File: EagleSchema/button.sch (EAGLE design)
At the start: 38 parts, among them IC1 TP4056

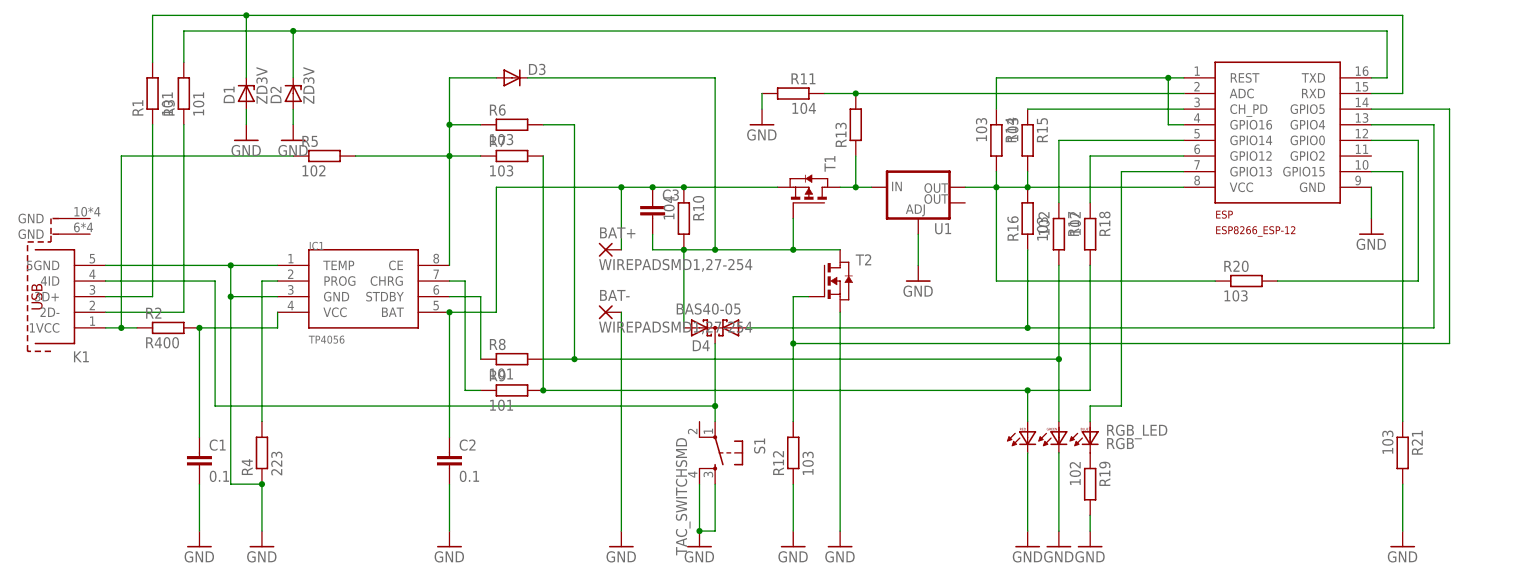
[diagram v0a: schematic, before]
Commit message: new version
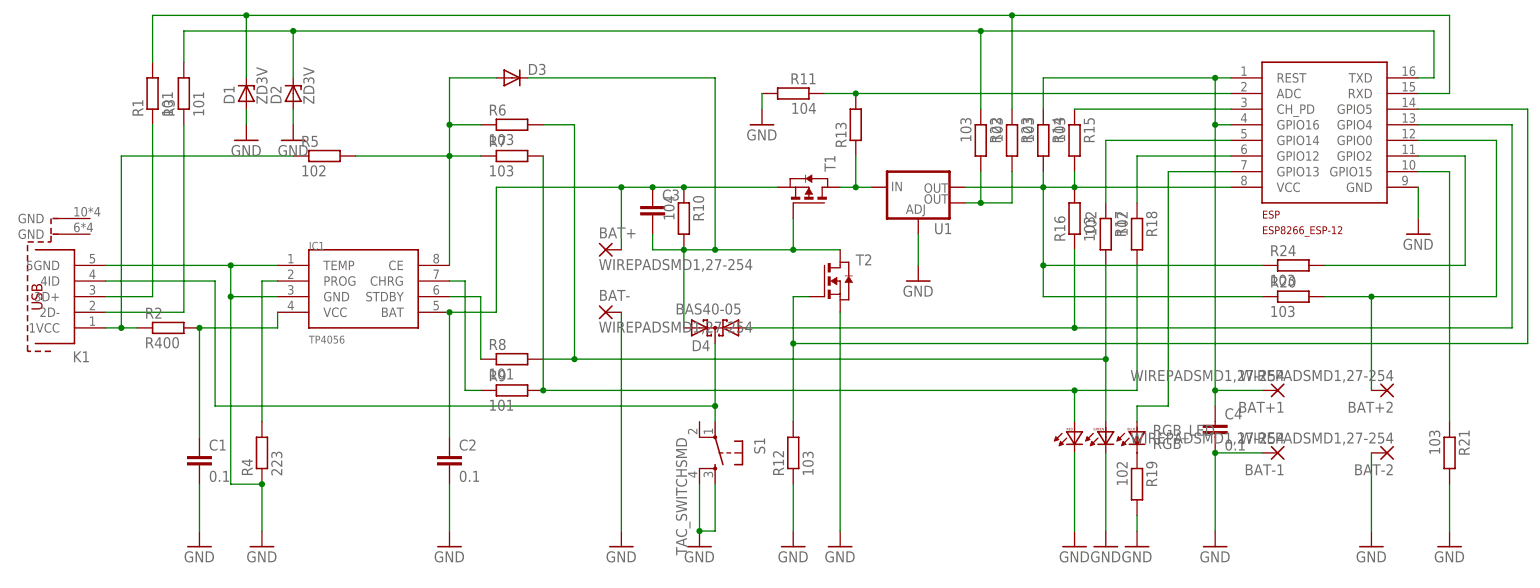
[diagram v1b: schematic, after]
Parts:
- added BAT+1, BAT+2, BAT-1, BAT-2: WIREPADSMD1,27-254, wirepad:WIREPADSMD1,27-254
- added C4: 0.1, resistor:C-EUC1206K
- added R22, R23, R24: 103, resistor:R-EU_R0603
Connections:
- new net N$17: ESP.GPIO2, R24.2
- new net N$29: R22.2, R23.2, U1.OUT@1
- net GND: now also BAT-1.P, BAT-2.P, C4.2
- net N$10: now also BAT+2.P
- net N$12: now also R24.1
- net N$27: now also R23.1
- net N$28: now also R22.1
- net N$7: now also BAT+1.P, C4.1
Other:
- moved on the sheet: ESP, R14, R15, R16, R17, R18, R19, R20, R21, RGB_LED
